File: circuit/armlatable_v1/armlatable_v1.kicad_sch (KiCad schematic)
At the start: 24 parts, among them J1 Conn_01x02_Pin, J2 Xiao ESP32S3, J3 Conn_01x04_Socket, J4 Conn_01x04_Socket, J6 Conn_01x02_Socket, J7 Conn_01x02_Socket, Q1 Q_Dual_PMOS_S1G1S2G2D2D2D1D1, SW1 SW_SPDT, U1 TSR0.5-2450, U2 MAX485E

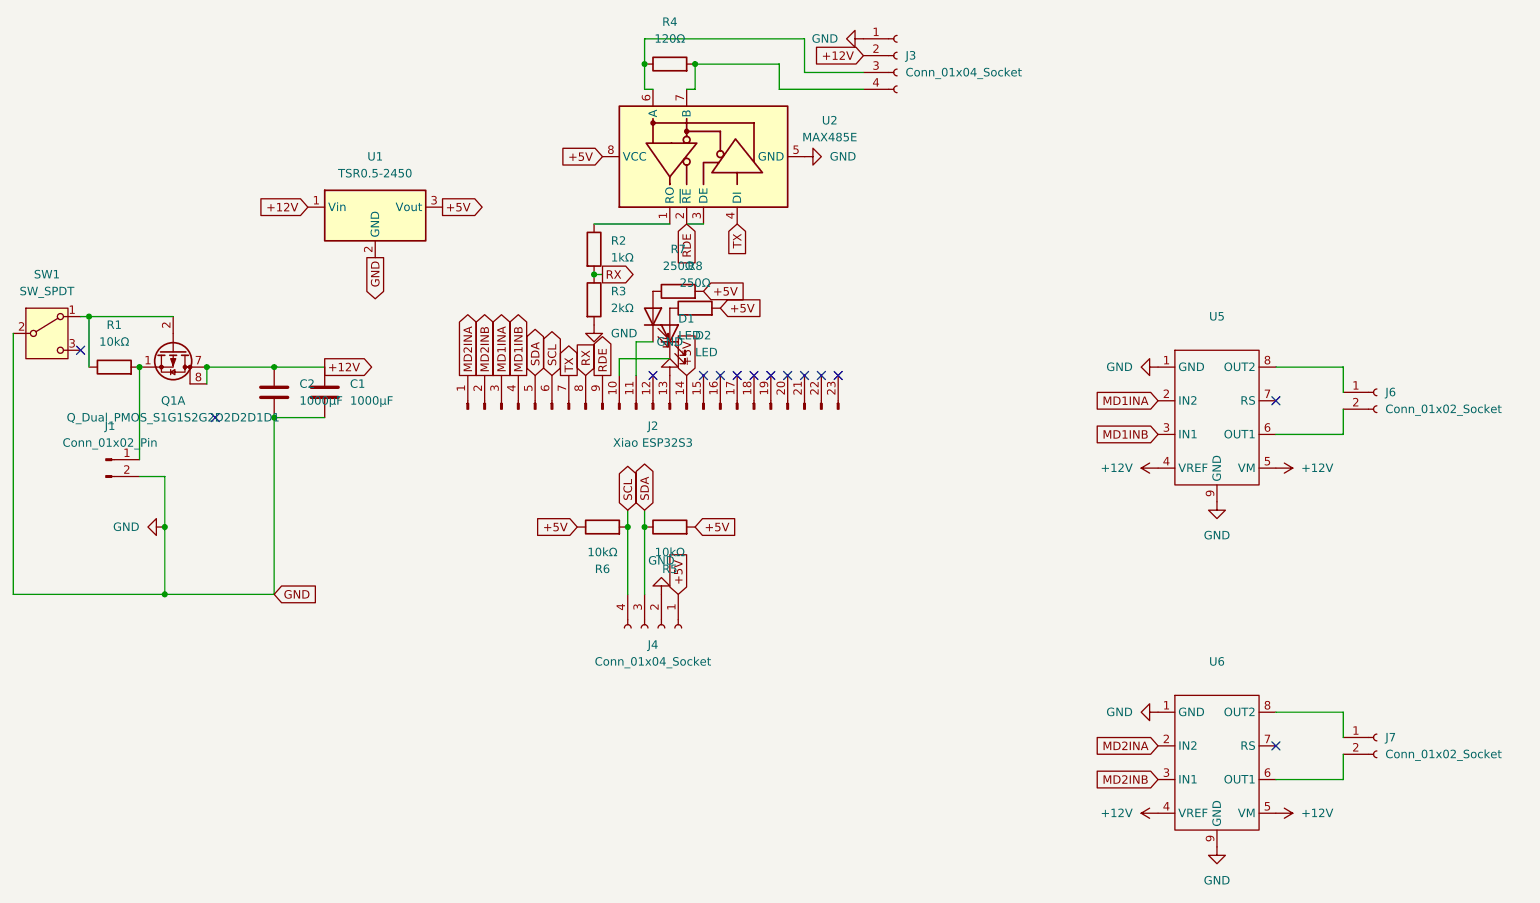
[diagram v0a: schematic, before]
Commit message: fix: Modify circuit
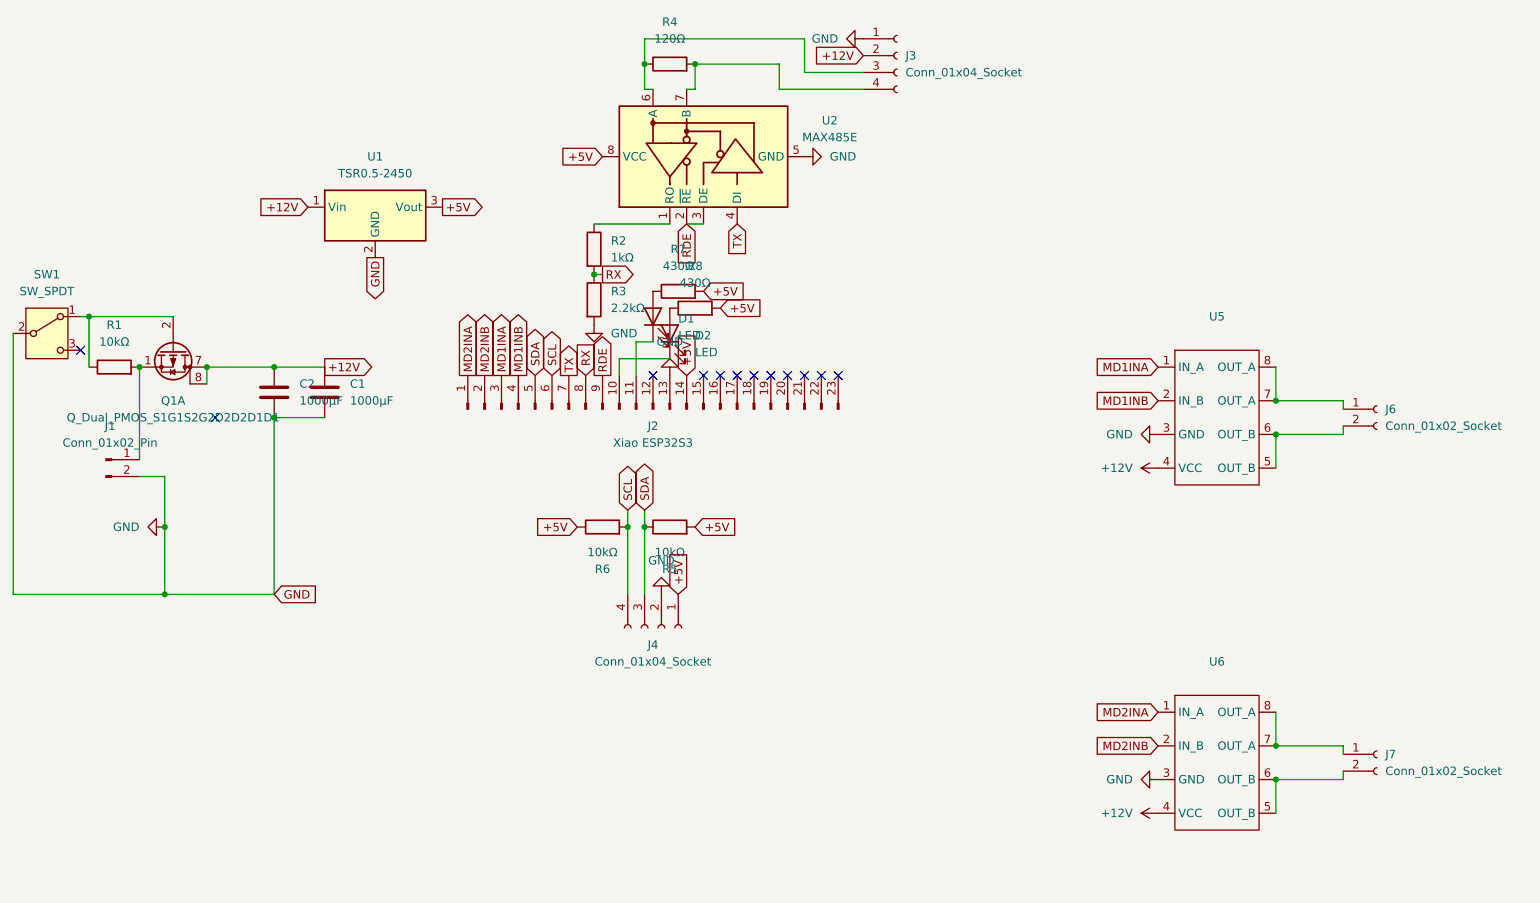
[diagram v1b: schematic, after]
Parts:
- R3: value 2kΩ -> 2.2kΩ
- R7, R8: value 250Ω -> 430Ω
- U5, U6: footprint Package_SO:HSOP-8-1EP_3.9x4.9mm_P1.27mm_EP2.41x3.1mm -> Package_SO:SO-8_3.9x4.9mm_P1.27mm; symbol custom:TB67H450FNG -> custom:AM2837
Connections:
- net +12V: no longer U5.5 (VM), U6.5 (VM)
- net GND: now also U5.3 (GND), U6.3 (GND); no longer U5.1 (GND), U5.9 (GND), U6.1 (GND), U6.9 (GND)
- net MD1INA: now also U5.1 (IN_A); no longer U5.2 (IN2)
- net MD1INB: now also U5.2 (IN_B); no longer U5.3 (IN1)
- net MD2INA: now also U6.1 (IN_A); no longer U6.2 (IN2)
- net MD2INB: now also U6.2 (IN_B); no longer U6.3 (IN1)
- net at J7.1 (Pin_1), U6.8 (OUT_A): now also U6.7 (OUT_A)
- net at J7.2 (Pin_2), U6.6 (OUT_B): now also U6.5 (OUT_B)
- net at J6.2 (Pin_2), U5.6 (OUT_B): now also U5.5 (OUT_B)
- net at U5.7 (OUT_A): now also J6.1 (Pin_1), U5.8 (OUT_A)
- no-connect marks 14 -> 12
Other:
- moved on the sheet: J6, J7
